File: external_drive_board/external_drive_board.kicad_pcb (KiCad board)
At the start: 2 copper layers, 90 x 90 mm, 33 parts, among them J1 MD-90SM, J2 MD-90SM, J3 Conn_02x17_Odd_Even, J4 Conn_01x04, J5 Conn_01x03, J7 Conn_01x03, SW1 SW_DIP_x08, U1 74LS125, U2 74LS85, U3 74LS595, U4 74LS165, U5 74LS04, U6 74LS165

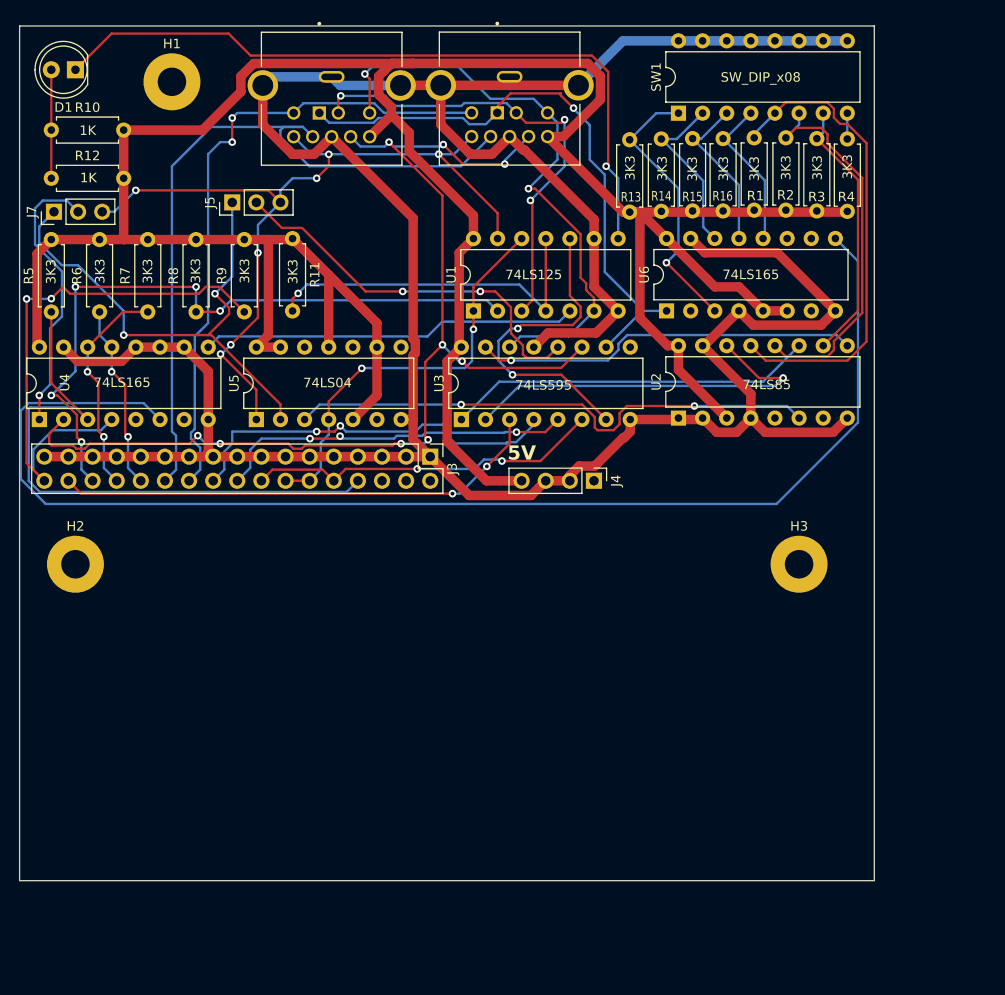
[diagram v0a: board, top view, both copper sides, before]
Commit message: finish M1565 initial board rev
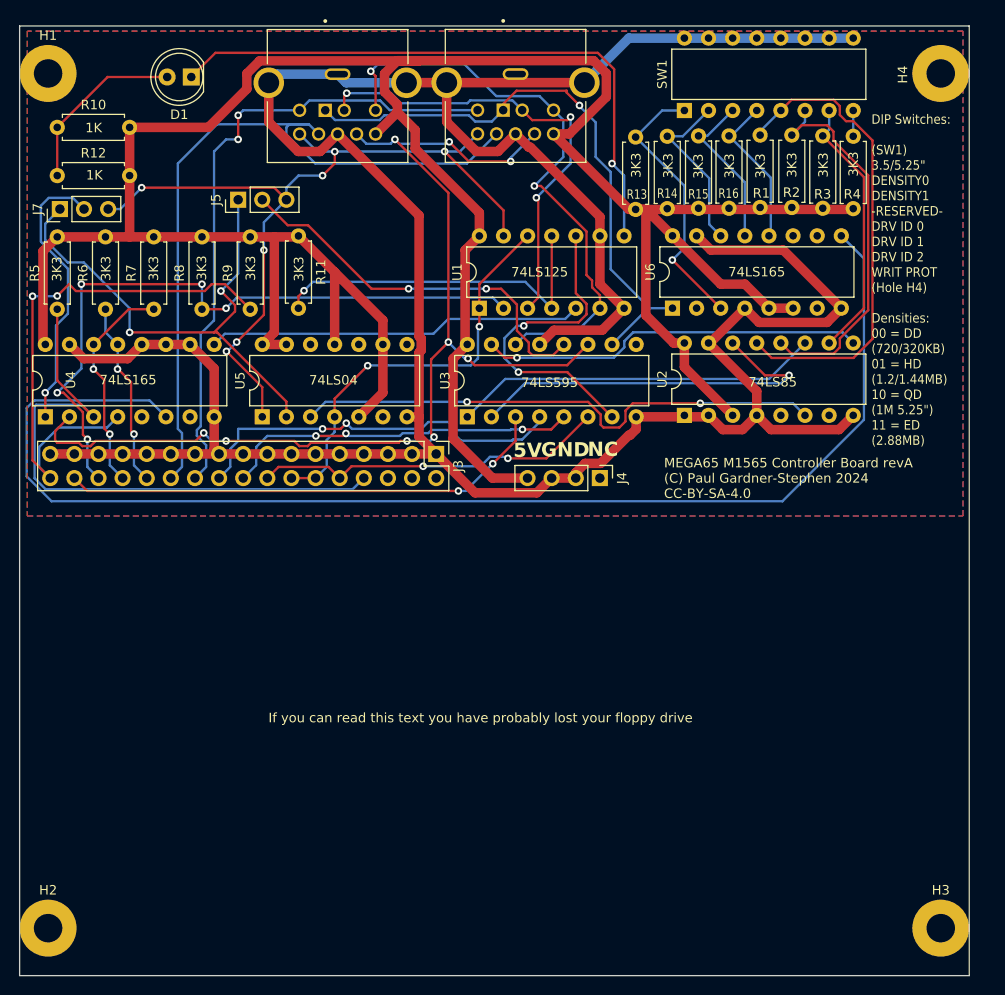
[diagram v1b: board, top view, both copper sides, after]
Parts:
- added H4: MountingHole, MountingHole:MountingHole_3mm_Pad, F.Cu at (147.0, 55.0)
- SW1: value SW_DIP_x08 -> SW_DIP_x04
- moved H3 41.1 mm to (147.0, 145.0)
- moved H2 38.4 mm to (53.0, 145.0)
- moved H1 13.1 mm to (53.0, 55.0)
- moved D1 12.2 mm to (68.1, 55.4)
- moved R2 0.68 mm to (131.3, 61.5)
- moved R4 0.68 mm to (137.8, 61.6)
- moved J3 0.68 mm to (93.9, 95.1)
- moved R1 0.68 mm to (128.0, 61.5)
- moved R14 0.68 mm to (118.2, 61.6)
- moved SW1 0.68 mm to (120.0, 58.9)
- moved J1 0.68 mm to (102.2, 55.1)
- moved J2 0.68 mm to (83.5, 55.1)
- moved J4 0.68 mm to (111.1, 97.6)
- moved J5 0.68 mm to (73.0, 68.3)
- moved J7 0.68 mm to (54.2, 69.3)
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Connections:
- net DIPSW3 renamed DENSITY1
- net DRIVE_HD renamed DENSITY0
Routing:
- net Net-(D1-K): track 77.5 -> 64.5 mm
- net Net-(D1-A): track 11.4 -> 18.9 mm
- added copper zone on B.Cu, net GND
- added copper zone on F.Cu, net GND
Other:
- board size 90 x 90 mm -> 100 x 100 mm
- board text added: "DIP Switches: (SW1) 3.5/5.25{dblquote} DENSITY0 DENSITY1 -RESERVED- DRV ID 0 DRV ID 1 DRV ID 2 WRIT PROT (Hole H4) Densities: 00 = DD (720/320KB) 01 = HD (1.2/1.44MB) 10 = QD (1M 5.25{dblquote}) 11 = ED (2.88MB)"
- board text added: "If you can read this text you have probably lost your floppy drive"
- board text added: "MEGA65 M1565 Controller Board revA (C) Paul Gardner-Stephen 2024 CC-BY-SA-4.0"
- board text added: "The floppy drive goes on the other side."
